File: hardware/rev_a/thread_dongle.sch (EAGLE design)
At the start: 24 parts, among them J1 USB-A-MALE-PLUG, J2 TC2030-JLINK-NL, U1 KW21Z, U2 ESDR0502N, U3 CP2102N-20, X1 FA-128, X2 FA-135

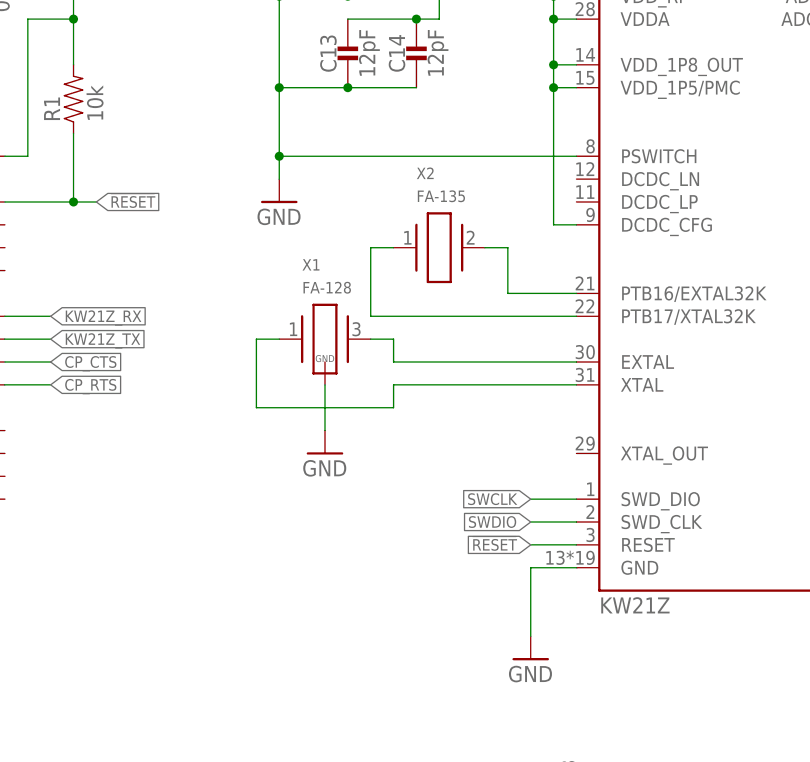
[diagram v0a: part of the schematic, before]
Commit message: Nothing to do and no errors
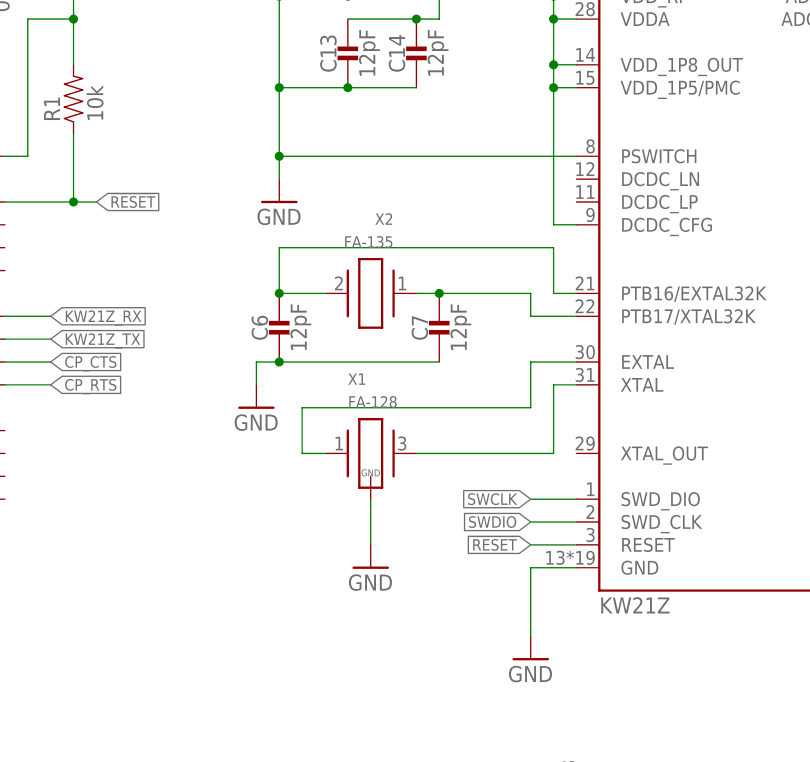
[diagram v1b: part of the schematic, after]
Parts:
- added C6, C7: 12pF, passives:CAPACITOR0402_CAP
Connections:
- removed net N$11: U1.EXTAL, X1.2
- removed net N$14: U1.PTB17/XTAL32K, X2.1
- removed net N$15: U1.PTB16/EXTAL32K, X2.2
- new net N$1: C6.1, U1.PTB16/EXTAL32K, X2.2
- new net N$2: C7.1, U1.PTB17/XTAL32K, X2.1
- new net N$3: U1.XTAL, X1.2
- net GND: now also C6.2, C7.2
- net N$12: now also U1.EXTAL; no longer U1.XTAL
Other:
- note added: "C10, C11, C12 place close to pin 20, 44, 28"
- note added: "C13, C14 place close to pins 36, 35"
- moved on the sheet: X1, X2
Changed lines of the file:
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@@
 <part name="SJ1" library="headers" deviceset="SOLDERJUMPER" device="NC"/>
 <part name="SJ2" library="headers" deviceset="SOLDERJUMPER" device="NC"/>
+<part name="C6" library="passives" deviceset="CAPACITOR" device="0402_CAP" value="12pF">
+<attribute name="DIGIKEY" value="490-5924-1-ND"/>
+</part>
+<part name="C7" library="passives" deviceset="CAPACITOR" device="0402_CAP" value="12pF">
+<attribute name="DIGIKEY" value="490-5924-1-ND"/>
+</part>
+<part name="GND1" library="supply1" library_urn="urn:adsk.eagle:library:371" deviceset="GND" device=""/>
 </parts>
 <sheets>
@@
 <plain>
 <text x="88.9" y="73.66" size="1.016" layer="98" align="bottom-center">FLOWCONTROL ENABLE</text>
+<text x="152.4" y="177.8" size="1.016" layer="98">C10, C11, C12 place close to pin 20, 44, 28</text>
+<text x="152.4" y="154.94" size="1.016" layer="98">C13, C14 place close to pins 36, 35</text>
 </plain>
 <instances>
@@
 <instance part="P+5" gate="VCC" x="147.32" y="180.34"/>
 <instance part="GND8" gate="1" x="147.32" y="144.78"/>
-<instance part="X1" gate="G$1" x="152.4" y="129.54">
-<attribute name="DIGIKEY" x="152.4" y="129.54" size="1.778" layer="96" display="off"/>
-</instance>
-<instance part="X2" gate="G$1" x="165.1" y="139.7">
-<attribute name="DIGIKEY" x="165.1" y="139.7" size="1.778" layer="96" display="off"/>
-</instance>
-<instance part="GND11" gate="1" x="152.4" y="116.84"/>
+<instance part="X1" gate="G$1" x="157.48" y="116.84">
+<attribute name="DIGIKEY" x="157.48" y="116.84" size="1.778" layer="96" display="off"/>
+</instance>
+<instance part="X2" gate="G$1" x="157.48" y="134.62" rot="MR0">
+<attribute name="DIGIKEY" x="157.48" y="134.62" size="1.778" layer="96" rot="MR0" display="off"/>
+</instance>
+<instance part="GND11" gate="1" x="157.48" y="104.14"/>
 <instance part="L1" gate="G$1" x="231.14" y="106.68" rot="R270">
 <attribute name="DIGIKEY" x="231.14" y="106.68" size="1.778" layer="96" rot="R270" display="off"/>
@@
 <attribute name="NAME" x="86.36" y="63.5" size="1.778" layer="95"/>
 </instance>
+<instance part="C6" gate="G$1" x="147.32" y="132.08">
+<attribute name="DIGIKEY" x="147.32" y="132.08" size="1.778" layer="96" display="off"/>
+</instance>
+<instance part="C7" gate="G$1" x="165.1" y="132.08">
+<attribute name="DIGIKEY" x="165.1" y="132.08" size="1.778" layer="96" display="off"/>
+</instance>
+<instance part="GND1" gate="1" x="144.78" y="121.92"/>
 </instances>
 <busses>
@@
 <segment>
 <pinref part="X1" gate="G$1" pin="GND"/>
-<wire x1="152.4" y1="124.46" x2="152.4" y2="119.38" width="0.1524" layer="91"/>
+<wire x1="157.48" y1="111.76" x2="157.48" y2="106.68" width="0.1524" layer="91"/>
 <pinref part="GND11" gate="1" pin="GND"/>
 </segment>
@@
 <pinref part="GND13" gate="1" pin="GND"/>
 <wire x1="220.98" y1="99.06" x2="220.98" y2="96.52" width="0.1524" layer="91"/>
+</segment>
+<segment>
+<pinref part="C7" gate="G$1" pin="2"/>
+<pinref part="C6" gate="G$1" pin="2"/>
+<wire x1="165.1" y1="127" x2="147.32" y2="127" width="0.1524" layer="91"/>
+<junction x="147.32" y="127"/>
+<pinref part="GND1" gate="1" pin="GND"/>
+<wire x1="144.78" y1="124.46" x2="144.78" y2="127" width="0.1524" layer="91"/>
+<wire x1="144.78" y1="127" x2="147.32" y2="127" width="0.1524" layer="91"/>
 </segment>
 </net>
@@
 </segment>
 </net>
-<net name="N$11" class="0">
-<segment>
-<pinref part="X1" gate="G$1" pin="2"/>
-<wire x1="157.48" y1="129.54" x2="160.02" y2="129.54" width="0.1524" layer="91"/>
-<wire x1="160.02" y1="129.54" x2="160.02" y2="127" width="0.1524" layer="91"/>
+<net name="N$12" class="0">
+<segment>
+<pinref part="X1" gate="G$1" pin="1"/>
+<wire x1="149.86" y1="116.84" x2="152.4" y2="116.84" width="0.1524" layer="91"/>
+<wire x1="149.86" y1="116.84" x2="149.86" y2="121.92" width="0.1524" layer="91"/>
+<wire x1="149.86" y1="121.92" x2="175.26" y2="121.92" width="0.1524" layer="91"/>
+<wire x1="175.26" y1="121.92" x2="175.26" y2="127" width="0.1524" layer="91"/>
 <pinref part="U1" gate="G$1" pin="EXTAL"/>
-<wire x1="160.02" y1="127" x2="180.34" y2="127" width="0.1524" layer="91"/>
-</segment>
-</net>
-<net name="N$12" class="0">
-<segment>
-<pinref part="U1" gate="G$1" pin="XTAL"/>
-<wire x1="180.34" y1="124.46" x2="160.02" y2="124.46" width="0.1524" layer="91"/>
-<wire x1="160.02" y1="124.46" x2="160.02" y2="121.92" width="0.1524" layer="91"/>
-<wire x1="160.02" y1="121.92" x2="144.78" y2="121.92" width="0.1524" layer="91"/>
-<wire x1="144.78" y1="121.92" x2="144.78" y2="129.54" width="0.1524" layer="91"/>
-<pinref part="X1" gate="G$1" pin="1"/>
-<wire x1="144.78" y1="129.54" x2="147.32" y2="129.54" width="0.1524" layer="91"/>
-</segment>
-</net>
-<net name="N$14" class="0">
-<segment>
-<pinref part="U1" gate="G$1" pin="PTB17/XTAL32K"/>
-<wire x1="157.48" y1="132.08" x2="180.34" y2="132.08" width="0.1524" layer="91"/>
-<pinref part="X2" gate="G$1" pin="1"/>
-<wire x1="160.02" y1="139.7" x2="157.48" y2="139.7" width="0.1524" layer="91"/>
-<wire x1="157.48" y1="139.7" x2="157.48" y2="132.08" width="0.1524" layer="91"/>
-</segment>
-</net>
-<net name="N$15" class="0">
-<segment>
-<pinref part="U1" gate="G$1" pin="PTB16/EXTAL32K"/>
-<wire x1="180.34" y1="134.62" x2="172.72" y2="134.62" width="0.1524" layer="91"/>
-<wire x1="172.72" y1="134.62" x2="172.72" y2="139.7" width="0.1524" layer="91"/>
-<pinref part="X2" gate="G$1" pin="2"/>
-<wire x1="172.72" y1="139.7" x2="170.18" y2="139.7" width="0.1524" layer="91"/>
+<wire x1="175.26" y1="127" x2="180.34" y2="127" width="0.1524" layer="91"/>
 </segment>
 </net>
@@
 </segment>
 </net>
+<net name="N$1" class="0">
+<segment>
+<pinref part="C6" gate="G$1" pin="1"/>
+<pinref part="U1" gate="G$1" pin="PTB16/EXTAL32K"/>
+<wire x1="180.34" y1="134.62" x2="177.8" y2="134.62" width="0.1524" layer="91"/>
+<wire x1="177.8" y1="134.62" x2="177.8" y2="139.7" width="0.1524" layer="91"/>
+<wire x1="177.8" y1="139.7" x2="147.32" y2="139.7" width="0.1524" layer="91"/>
+<wire x1="147.32" y1="139.7" x2="147.32" y2="134.62" width="0.1524" layer="91"/>
+<pinref part="X2" gate="G$1" pin="2"/>
+<wire x1="152.4" y1="134.62" x2="147.32" y2="134.62" width="0.1524" layer="91"/>
+<junction x="147.32" y="134.62"/>
+</segment>
+</net>
+<net name="N$2" class="0">
+<segment>
+<pinref part="C7" gate="G$1" pin="1"/>
+<pinref part="U1" gate="G$1" pin="PTB17/XTAL32K"/>
+<wire x1="180.34" y1="132.08" x2="175.26" y2="132.08" width="0.1524" layer="91"/>
+<wire x1="175.26" y1="132.08" x2="175.26" y2="134.62" width="0.1524" layer="91"/>
+<wire x1="175.26" y1="134.62" x2="165.1" y2="134.62" width="0.1524" layer="91"/>
+<pinref part="X2" gate="G$1" pin="1"/>
+<wire x1="162.56" y1="134.62" x2="165.1" y2="134.62" width="0.1524" layer="91"/>
+<junction x="165.1" y="134.62"/>
+</segment>
+</net>
+<net name="N$3" class="0">
+<segment>
+<pinref part="U1" gate="G$1" pin="XTAL"/>
+<wire x1="180.34" y1="124.46" x2="177.8" y2="124.46" width="0.1524" layer="91"/>
+<wire x1="177.8" y1="124.46" x2="177.8" y2="116.84" width="0.1524" layer="91"/>
+<pinref part="X1" gate="G$1" pin="2"/>
+<wire x1="177.8" y1="116.84" x2="162.56" y2="116.84" width="0.1524" layer="91"/>
+</segment>
+</net>
